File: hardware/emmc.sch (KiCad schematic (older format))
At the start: 12 parts, among them U400 EMMC_BGA_153

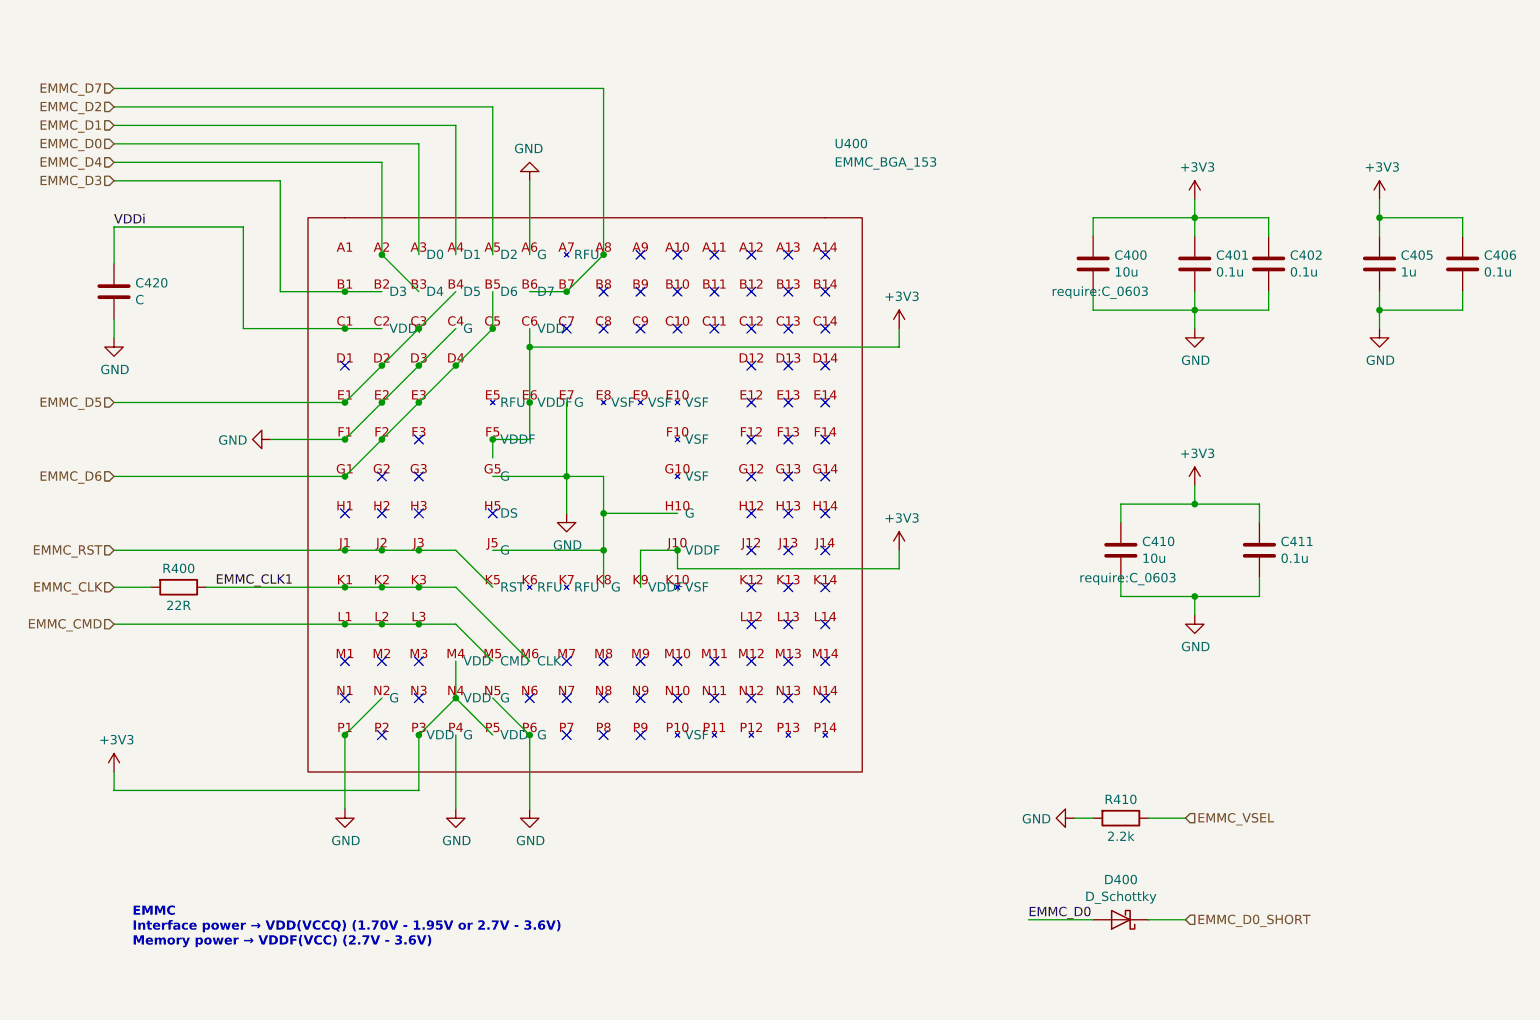
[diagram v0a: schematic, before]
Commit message: wip
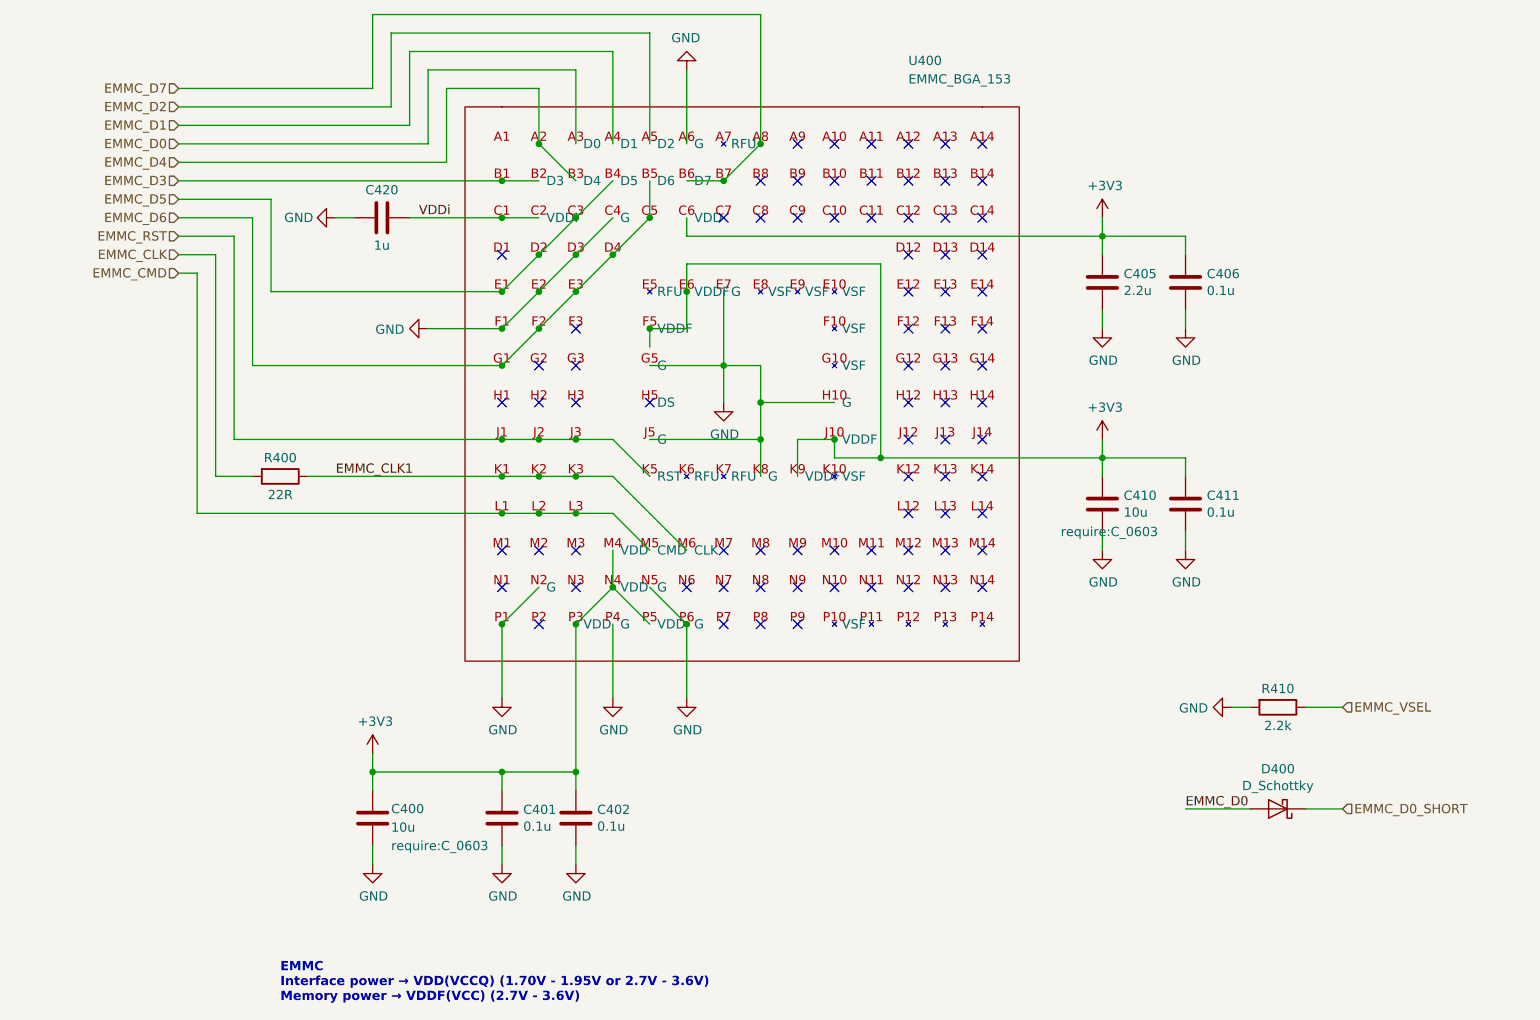
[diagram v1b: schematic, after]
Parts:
- C405: value 1u -> 2.2u
- C420: value C -> 1u
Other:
- moved on the sheet: C400, C401, C402, C405, C406, C410, C411, C420, D400, R400, R410, U400
